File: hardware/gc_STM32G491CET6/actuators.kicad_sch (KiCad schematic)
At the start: 37 parts, among them U401 NCS199A3RSQT2G, U402 NCS199A3RSQT2G, U403 ZXBM5210-S, U404 ZXBM5210-S

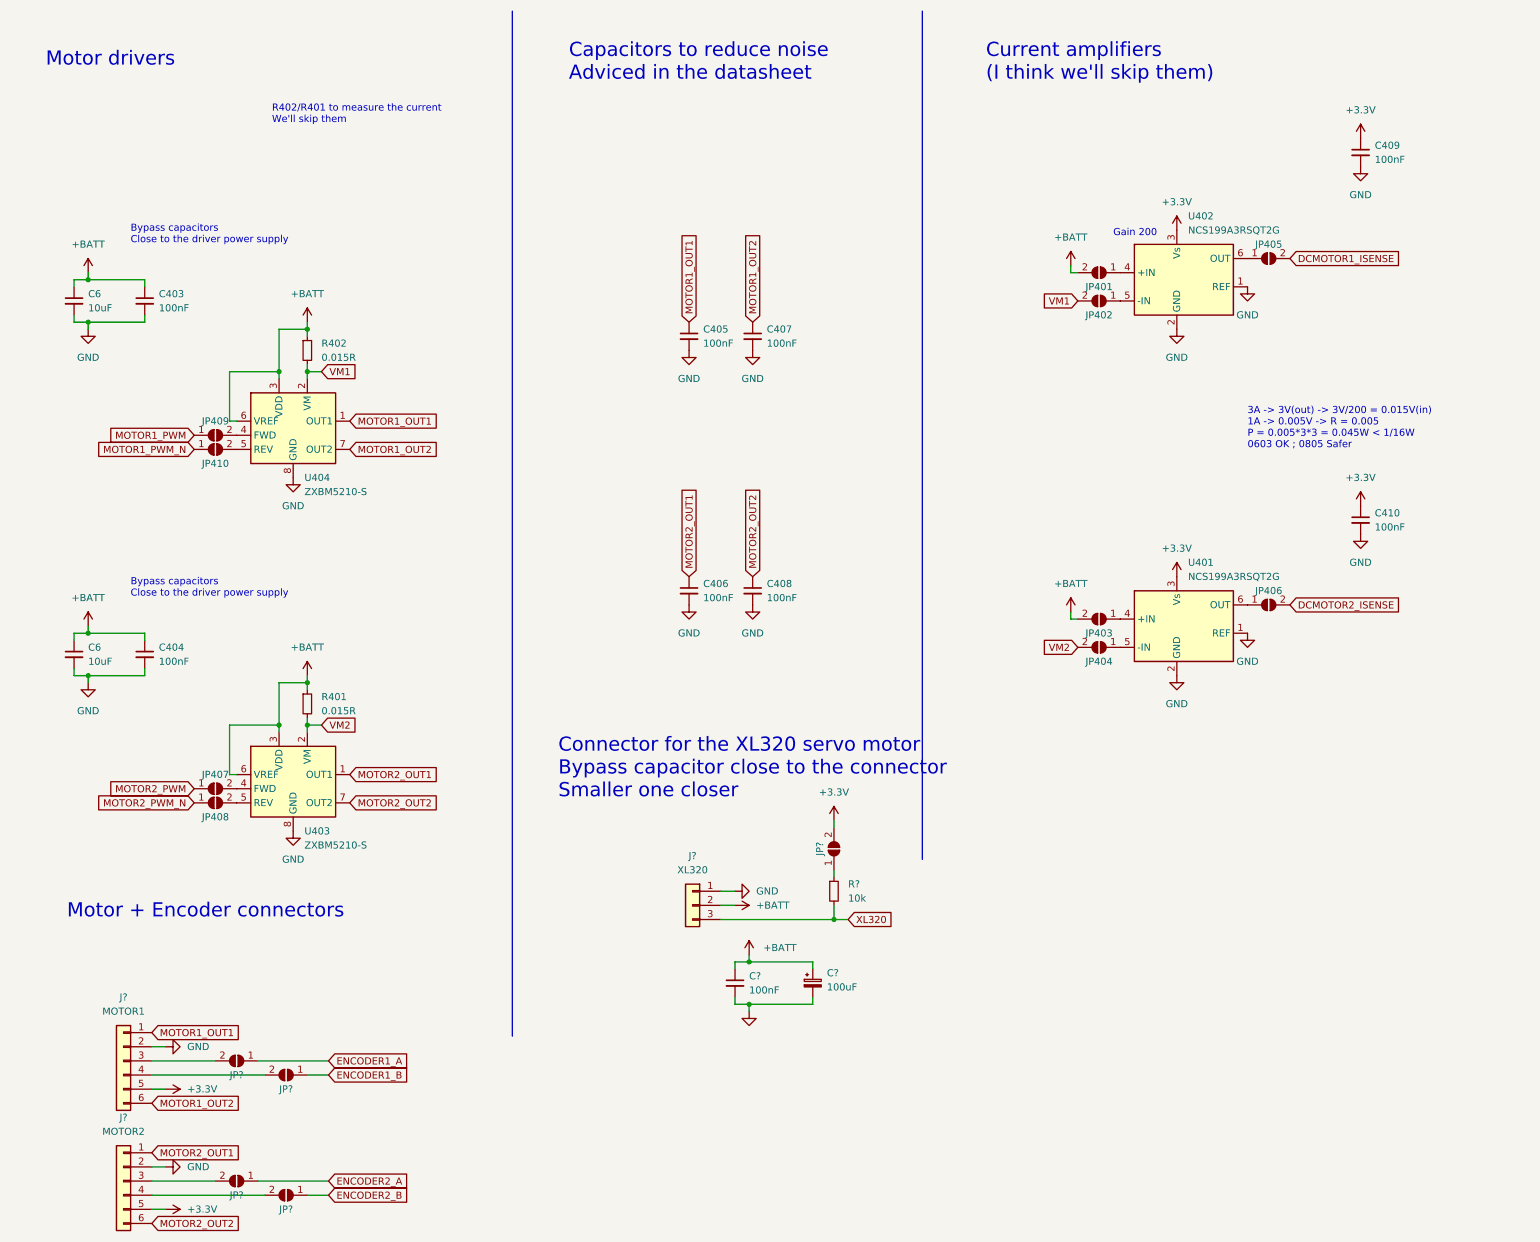
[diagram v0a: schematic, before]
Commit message: Schematics + rough placement
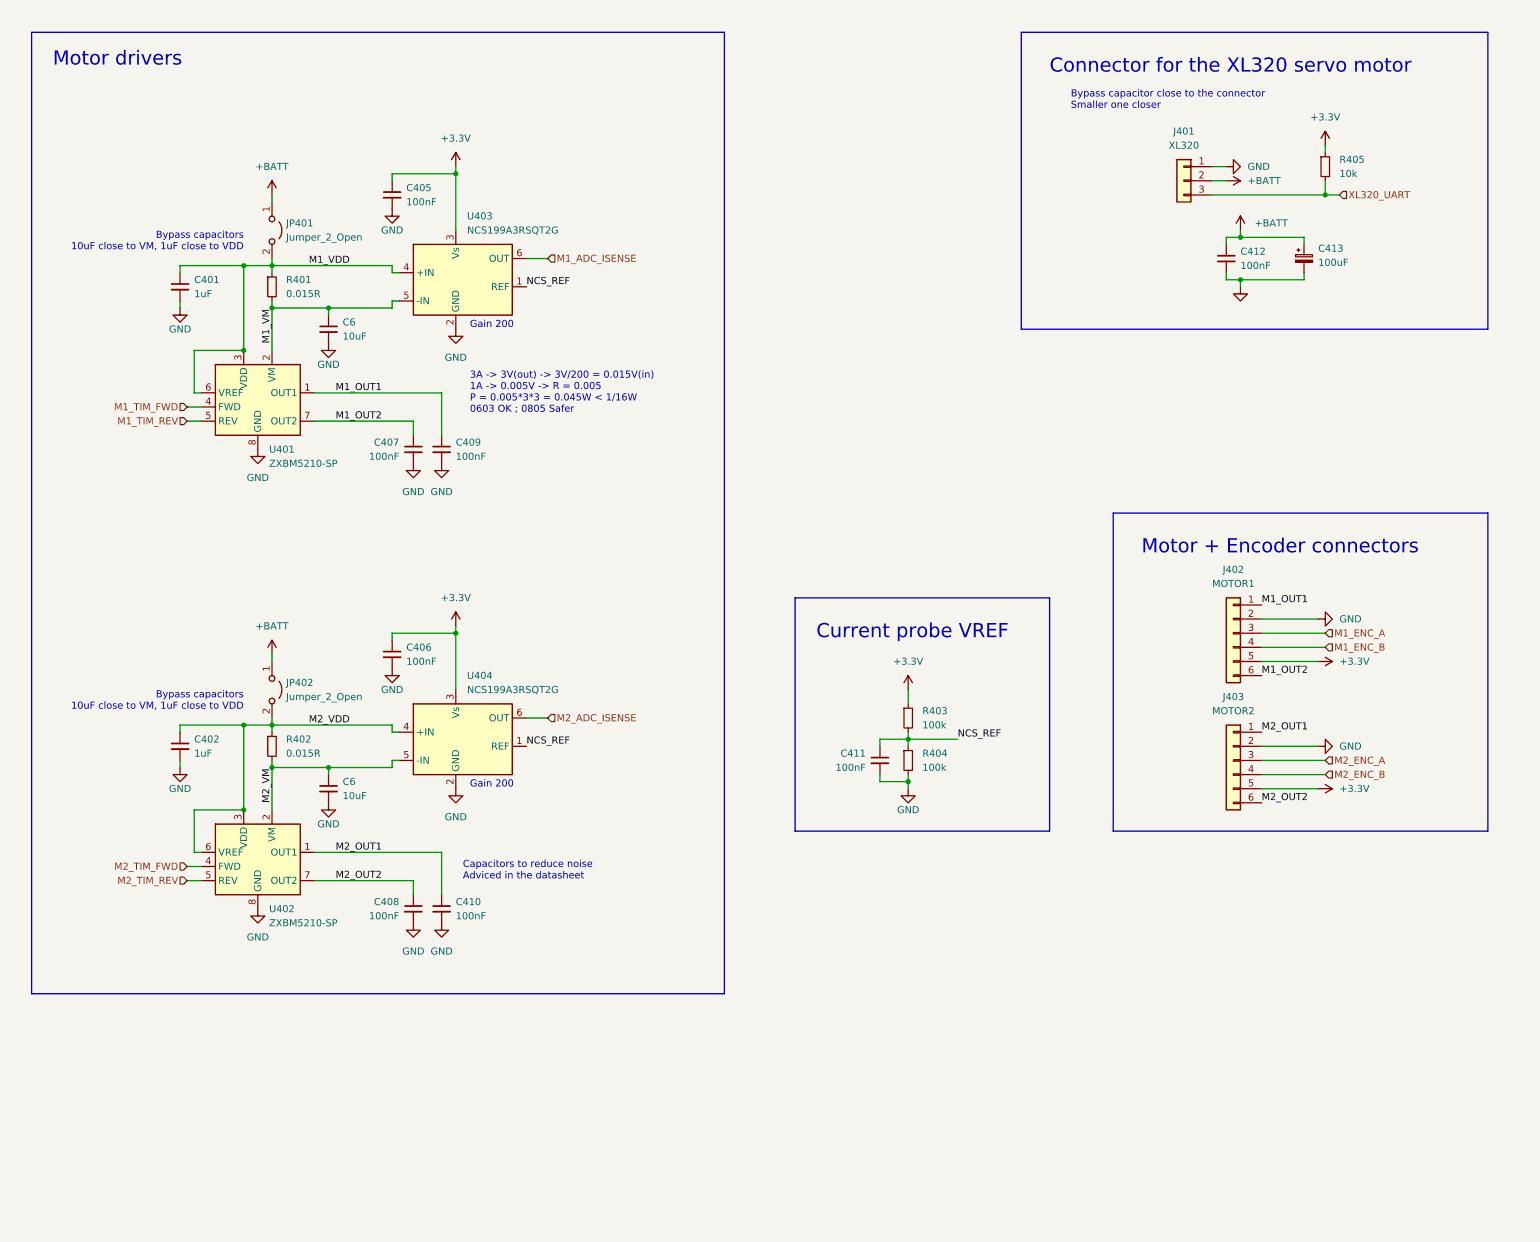
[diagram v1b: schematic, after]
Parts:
- removed C403: 100nF, Capacitor_SMD:C_0603_1608Metric_Pad1.08x0.95mm_HandSolder, symbol Device:C_Small
- removed JP401, JP402, JP403, JP404, JP405, JP406, JP407, JP408, JP409, JP410, JP? (x5): SolderJumper_2_Open, Jumper:SolderJumper-2_P1.3mm_Open_TrianglePad1.0x1.5mm, symbol Jumper:SolderJumper_2_Open
- removed R402: 0.015R, Resistor_SMD:R_0805_2012Metric_Pad1.20x1.40mm_HandSolder, symbol Device:R_Small
- removed U402: NCS199A3RSQT2G, Package_TO_SOT_SMD:SOT-363_SC-70-6_Handsoldering, symbol Amplifier_Current:NCS210
- removed U403, U404: ZXBM5210-S, Package_SO:SOIC-8_3.9x4.9mm_P1.27mm, symbol Driver_Motor:ZXBM5210-S
- added C401: 1uF, Capacitor_SMD:C_0603_1608Metric_Pad1.08x0.95mm_HandSolder, symbol Device:C_Small
- added C411: 100nF, Capacitor_SMD:C_0603_1608Metric_Pad1.08x0.95mm_HandSolder, symbol Device:C_Small
- added JP401, JP402: Jumper_2_Open, Connector_PinHeader_2.54mm:PinHeader_1x02_P2.54mm_Vertical, symbol Jumper:Jumper_2_Open
- added R401: 0.015R, Resistor_SMD:R_0805_2012Metric_Pad1.20x1.40mm_HandSolder, symbol Device:R_Small
- added R403, R404: 100k, Resistor_SMD:R_0603_1608Metric, symbol Device:R_Small
- added U401, U402: ZXBM5210-SP, Package_SO:Diodes_SO-8EP, symbol Driver_Motor:ZXBM5210-SP
- added U403: NCS199A3RSQT2G, Package_TO_SOT_SMD:SOT-363_SC-70-6, symbol Amplifier_Current:NCS210
- C402: renamed from C404; value 100nF -> 1uF
- U404: renamed from U401; footprint Package_TO_SOT_SMD:SOT-363_SC-70-6_Handsoldering -> Package_TO_SOT_SMD:SOT-363_SC-70-6
- gave numbers to parts that had none: 6
- renumbered C410 to C406, C406 to C408, C408 to C410, R401 to R402
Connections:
- net VM2 is gone; now on net M2_VM: R402.2
- net +BATT: now also JP401.1 (A), JP402.1 (A); no longer C402.1, C6.1, C6.1, R402.1
- net GND: now also C401.2, C411.2, R404.2, U401.8 (GND), U401.9 (GND), U402.8 (GND), U402.9 (GND), U403.2 (GND); no longer U404.1 (REF)
- net M1_ENC_B: now reaches J402.4 (Pin_4)
- net +3.3V: now reaches R405.1
- net +3.3V: now also C405.1, C406.1, J402.5 (Pin_5), J403.5 (Pin_5), U404.3 (Vs), R403.1, U403.3 (Vs)
- net M1_ENC_A: now reaches J402.3 (Pin_3)
- net M2_VDD: now reaches U404.4 (+IN)
- net M2_VDD: now also C402.1, R402.1, JP402.2 (B), U402.3 (VDD), U402.6 (VREF)
- net M2_VM: now reaches U404.5 (-IN)
- net M2_VM: now also C6.1, U402.2 (VM)
- net M2_ENC_A: now reaches J403.3 (Pin_3)
- net M2_ENC_B: now reaches J403.4 (Pin_4)
- net M2_ADC_ISENSE: now reaches U404.6 (OUT)
- removed net +3V3: C406.1, C409.1, J402.5 (Pin_5), J403.5 (Pin_5), U404.3 (Vs)
- net MOTOR1_OUT1 renamed M1_OUT1
- net M1_OUT1: now also C409.1, U401.1 (OUT1); no longer C405.1
- net MOTOR1_OUT2 renamed M1_OUT2
- net M1_OUT2: now also U401.7 (OUT2)
- net MOTOR2_OUT1 renamed M2_OUT1
- net M2_OUT1: now also C410.1, U402.1 (OUT1); no longer C408.1
- net MOTOR2_OUT2 renamed M2_OUT2
- net M2_OUT2: now also C408.1, U402.7 (OUT2); no longer C410.1
- net XL320 renamed XL320_UART
- new net M1_ADC_ISENSE: U403.6 (OUT)
- new net M1_TIM_FWD: U401.4 (FWD)
- new net M1_TIM_REV: U401.5 (REV)
- new net M1_VDD: C401.1, JP401.2 (B), R401.1, U401.3 (VDD), U401.6 (VREF), U403.4 (+IN)
- new net M1_VM: C6.1, R401.2, U401.2 (VM), U403.5 (-IN)
- new net M2_TIM_FWD: U402.4 (FWD)
- new net M2_TIM_REV: U402.5 (REV)
- new net NCS_REF: C411.1, R403.2, R404.1, U403.1 (REF), U404.1 (REF)
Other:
- note added: "Bypass capacitor close to the connector Smaller one closer"
- note added: "Bypass capacitors 10uF close to VM, 1uF close to VDD"
- note added: "Connector for the XL320 servo motor"
- note added: "Current probe VREF"
- note removed: "Bypass capacitors Close to the driver power supply"
- note removed: "Connector for the XL320 servo motor Bypass capacitor close to the connector Smaller one closer"
- note removed: "Current amplifiers (I think we'll skip them)"
- note removed: "R402/R401 to measure the current We'll skip them"
- moved on the sheet: C402, C406, C408, C410, C412, C413, C6, J401, J402, J403, R402, R405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

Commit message: placement
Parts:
- C401, C402, C405, C406, C407, C408, C409, C410, C411, C412: footprint Capacitor_SMD:C_0603_1608Metric_Pad1.08x0.95mm_HandSolder -> Capacitor_SMD:C_0603_1608Metric
- R401, R402: footprint Resistor_SMD:R_0805_2012Metric_Pad1.20x1.40mm_HandSolder -> Resistor_SMD:R_0805_2012Metric
- R405: footprint Resistor_SMD:R_0603_1608Metric_Pad0.98x0.95mm_HandSolder -> Resistor_SMD:R_0603_1608Metric
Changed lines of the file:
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@@
       (effects (font (size 1.27 1.27)) (justify left))
     )
-    (property "Footprint" "Capacitor_SMD:C_0603_1608Metric_Pad1.08x0.95mm_HandSolder" (id 2) (at 90.17 91.44 0)
+    (property "Footprint" "Capacitor_SMD:C_0603_1608Metric" (id 2) (at 90.17 91.44 0)
       (effects (font (size 1.27 1.27)) hide)
     )
@@
       (effects (font (size 1.27 1.27)) (justify left))
     )
-    (property "Footprint" "Capacitor_SMD:C_0603_1608Metric_Pad1.08x0.95mm_HandSolder" (id 2) (at 231.14 57.15 0)
+    (property "Footprint" "Capacitor_SMD:C_0603_1608Metric" (id 2) (at 231.14 57.15 0)
       (effects (font (size 1.27 1.27)) hide)
     )
@@
       (effects (font (size 1.27 1.27)) (justify left))
     )
-    (property "Footprint" "Capacitor_SMD:C_0603_1608Metric_Pad1.08x0.95mm_HandSolder" (id 2) (at 168.91 147.32 0)
+    (property "Footprint" "Capacitor_SMD:C_0603_1608Metric" (id 2) (at 168.91 147.32 0)
       (effects (font (size 1.27 1.27)) hide)
     )
@@
       (effects (font (size 1.27 1.27)) (justify right))
     )
-    (property "Footprint" "Capacitor_SMD:C_0603_1608Metric_Pad1.08x0.95mm_HandSolder" (id 2) (at 85.09 173.99 0)
+    (property "Footprint" "Capacitor_SMD:C_0603_1608Metric" (id 2) (at 85.09 173.99 0)
       (effects (font (size 1.27 1.27)) hide)
     )
@@
       (effects (font (size 1.27 1.27)) (justify left))
     )
-    (property "Footprint" "Capacitor_SMD:C_0603_1608Metric_Pad1.08x0.95mm_HandSolder" (id 2) (at 69.85 69.85 0)
+    (property "Footprint" "Capacitor_SMD:C_0603_1608Metric" (id 2) (at 69.85 69.85 0)
       (effects (font (size 1.27 1.27)) hide)
     )
@@
       (effects (font (size 1.27 1.27)) (justify left))
     )
-    (property "Footprint" "Capacitor_SMD:C_0603_1608Metric_Pad1.08x0.95mm_HandSolder" (id 2) (at 69.85 152.4 0)
+    (property "Footprint" "Capacitor_SMD:C_0603_1608Metric" (id 2) (at 69.85 152.4 0)
       (effects (font (size 1.27 1.27)) hide)
     )
@@
       (effects (font (size 1.27 1.27)) (justify left))
     )
-    (property "Footprint" "Resistor_SMD:R_0603_1608Metric_Pad0.98x0.95mm_HandSolder" (id 2) (at 248.92 40.64 0)
+    (property "Footprint" "Resistor_SMD:R_0603_1608Metric" (id 2) (at 248.92 40.64 0)
       (effects (font (size 1.27 1.27)) hide)
     )
@@
       (effects (font (size 1.27 1.27)) (justify left))
     )
-    (property "Footprint" "Resistor_SMD:R_0805_2012Metric_Pad1.20x1.40mm_HandSolder" (id 2) (at 59.69 62.23 0)
+    (property "Footprint" "Resistor_SMD:R_0805_2012Metric" (id 2) (at 59.69 62.23 0)
       (effects (font (size 1.27 1.27)) hide)
     )
@@
       (effects (font (size 1.27 1.27)) (justify left))
     )
-    (property "Footprint" "Resistor_SMD:R_0805_2012Metric_Pad1.20x1.40mm_HandSolder" (id 2) (at 59.69 144.78 0)
+    (property "Footprint" "Resistor_SMD:R_0805_2012Metric" (id 2) (at 59.69 144.78 0)
       (effects (font (size 1.27 1.27)) hide)
     )
@@
       (effects (font (size 1.27 1.27)) (justify right))
     )
-    (property "Footprint" "Capacitor_SMD:C_0603_1608Metric_Pad1.08x0.95mm_HandSolder" (id 2) (at 85.09 91.44 0)
+    (property "Footprint" "Capacitor_SMD:C_0603_1608Metric" (id 2) (at 85.09 91.44 0)
       (effects (font (size 1.27 1.27)) hide)
     )
@@
       (effects (font (size 1.27 1.27)) (justify left))
     )
-    (property "Footprint" "Capacitor_SMD:C_0603_1608Metric_Pad1.08x0.95mm_HandSolder" (id 2) (at 81.28 45.72 0)
+    (property "Footprint" "Capacitor_SMD:C_0603_1608Metric" (id 2) (at 81.28 45.72 0)
       (effects (font (size 1.27 1.27)) hide)
     )
@@
       (effects (font (size 1.27 1.27)) (justify left))
     )
-    (property "Footprint" "Capacitor_SMD:C_0603_1608Metric_Pad1.08x0.95mm_HandSolder" (id 2) (at 90.17 173.99 0)
+    (property "Footprint" "Capacitor_SMD:C_0603_1608Metric" (id 2) (at 90.17 173.99 0)
       (effects (font (size 1.27 1.27)) hide)
     )
@@
       (effects (font (size 1.27 1.27)) (justify left))
     )
-    (property "Footprint" "Capacitor_SMD:C_0603_1608Metric_Pad1.08x0.95mm_HandSolder" (id 2) (at 43.18 62.23 0)
+    (property "Footprint" "Capacitor_SMD:C_0603_1608Metric" (id 2) (at 43.18 62.23 0)
       (effects (font (size 1.27 1.27)) hide)
     )
@@
       (effects (font (size 1.27 1.27)) (justify left))
     )
-    (property "Footprint" "Capacitor_SMD:C_0603_1608Metric_Pad1.08x0.95mm_HandSolder" (id 2) (at 81.28 128.27 0)
+    (property "Footprint" "Capacitor_SMD:C_0603_1608Metric" (id 2) (at 81.28 128.27 0)
       (effects (font (size 1.27 1.27)) hide)
     )
@@
       (effects (font (size 1.27 1.27)) (justify left))
     )
-    (property "Footprint" "Capacitor_SMD:C_0603_1608Metric_Pad1.08x0.95mm_HandSolder" (id 2) (at 43.18 144.78 0)
-      (effects (font (size 1.27 1.27)) hide)
-    )
+    (property "Footprint" "Capacitor_SMD:C_0603_1608Metric" (id 2) (at 43.18 144.78 0)
+      (effects (font (size 1.27 1.27)) hide)
+    )
